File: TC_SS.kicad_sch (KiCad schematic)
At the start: 25 parts, among them J1 Conn_01x08_Pin, J2 Conn_01x08_Pin, Q1 IPW60R099P6XKSA1, Q2 IPW60R099P6XKSA1, Q3 IPW60R099P6XKSA1, Q4 IPW60R099P6XKSA1

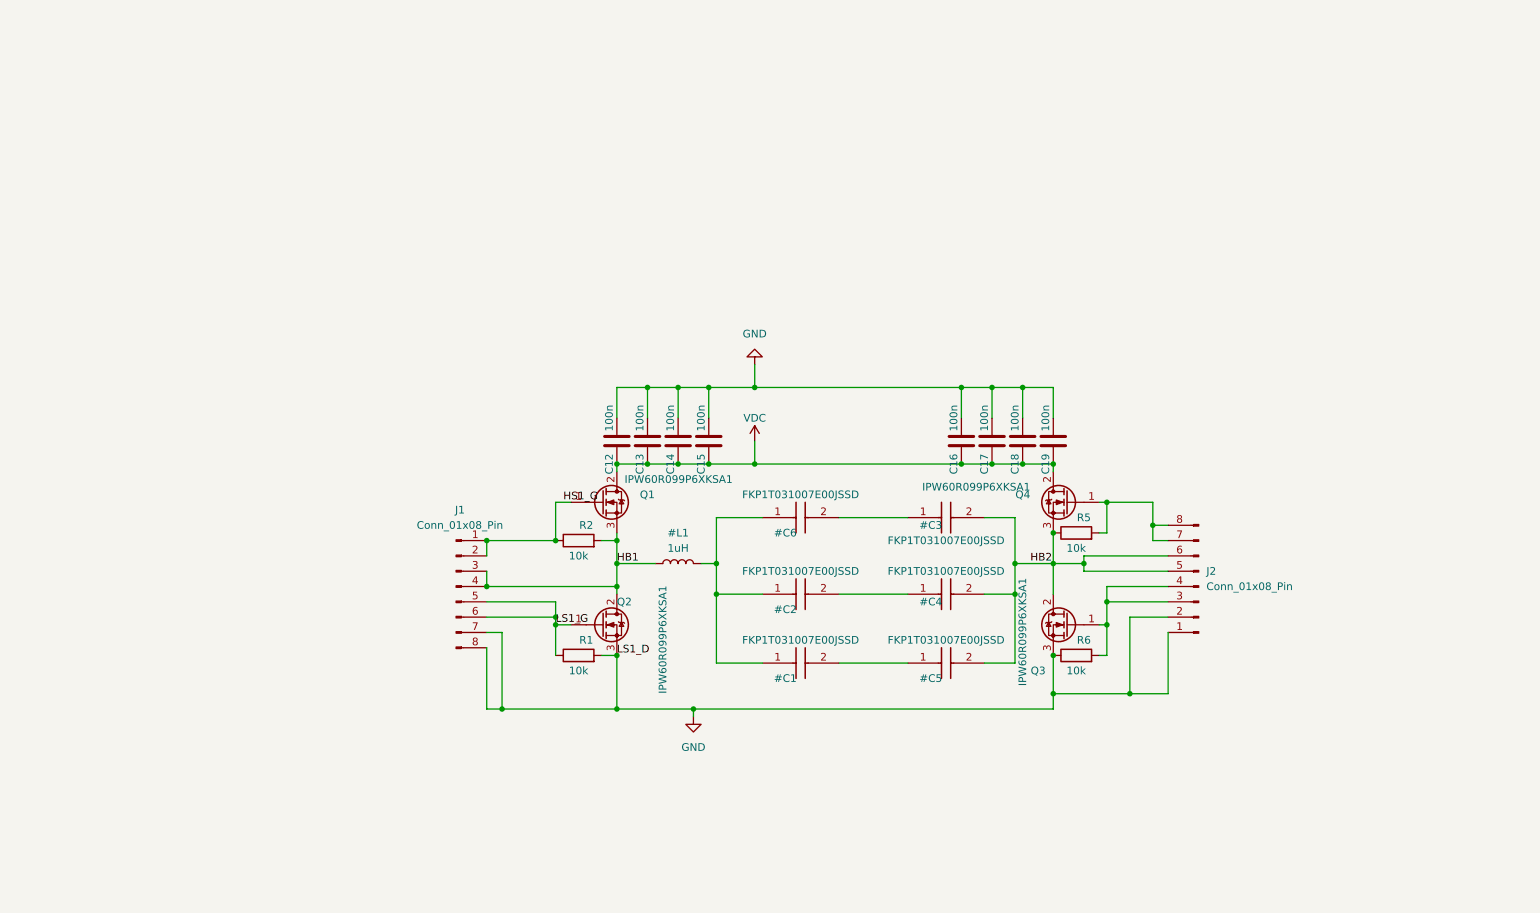
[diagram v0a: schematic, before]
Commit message: Update basically everything
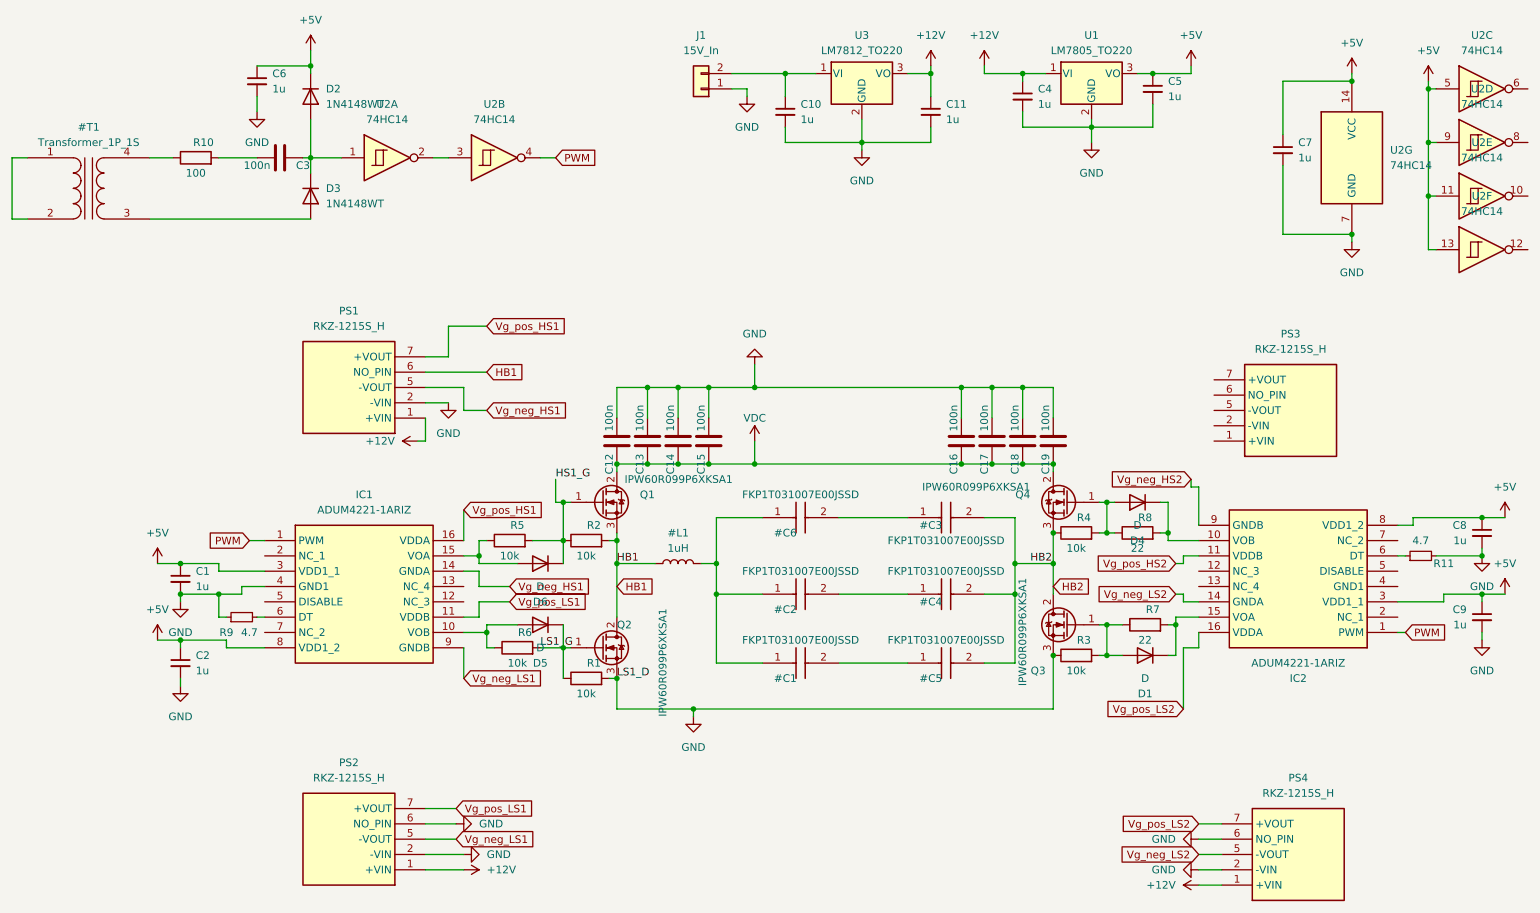
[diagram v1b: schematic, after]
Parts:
- removed J1, J2: Conn_01x08_Pin, Connector_PinHeader_2.54mm:PinHeader_1x08_P2.54mm_Vertical, symbol Connector:Conn_01x08_Pin
- added #T1: Transformer_1P_1S, symbol Device:Transformer_1P_1S
- added C1, C10, C11, C2, C4, C5, C6, C7, C8, C9: 1u, Capacitor_SMD:C_0805_2012Metric, symbol Device:C_Small
- added C3: 100n, Capacitor_SMD:C_2220_5650Metric, symbol Device:C
- added D1, D4, D5, D6: D, PCM_Diode_SMD_AKL:D_PowerDI-123, symbol Device:D
- added D2, D3: 1N4148WT, Diode_SMD:D_SOD-523, symbol Diode:1N4148WT
- added IC1, IC2: ADUM4221-1ARIZ, SamacSys_Parts:SOIC127P1030X264-16N, symbol SamacSys_Parts:ADUM4221-1ARIZ
- added J1: 15V_In, Connector_PinHeader_2.54mm:PinHeader_1x02_P2.54mm_Vertical, symbol Connector_Generic:Conn_01x02
- added PS1, PS2, PS3, PS4: RKZ-1215S_H, symbol:RKZ1215SH, symbol SamacSys_Parts:RKZ-1215S_H
- added R10: 100, Resistor_SMD:R_0805_2012Metric, symbol Device:R
- added R11, R9: 4.7, Resistor_SMD:R_0805_2012Metric, symbol Device:R_Small
- added R3, R4: 10k, Resistor_SMD:R_0805_2012Metric, symbol Device:R
- added R7, R8: 22, Resistor_SMD:R_0805_2012Metric, symbol Device:R
- added U1: LM7805_TO220, Package_TO_SOT_THT:TO-220-3_Vertical, symbol Regulator_Linear:LM7805_TO220
- added U2: 74HC14, symbol 74xx:74HC14
- added U3: LM7812_TO220, Package_TO_SOT_THT:TO-220-3_Vertical, symbol Regulator_Linear:LM7812_TO220
- R1, R2, R5, R6: footprint Resistor_SMD:R_1206_3216Metric_Pad1.30x1.75mm_HandSolder -> Resistor_SMD:R_0805_2012Metric
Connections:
- net GND: now also C1.2, C10.2, C11.2, C2.2, C4.2, C5.2, C6.2, C7.2, C8.2, C9.2, IC1.4 (GND1), J1.1 (Pin_1), PS1.2 (-VIN), PS2.2 (-VIN), PS2.6 (NO_PIN), PS4.2 (-VIN), PS4.6 (NO_PIN), R11.2, R3.1, R9.1, U1.2 (GND), U2.7 (GND), U3.2 (GND); no longer R6.1
- net HB1: now also PS1.6 (NO_PIN)
- net HB2: now also R4.1; no longer R5.1
- net HS1_G: now also R5.2, D6.1 (K)
- net LS1_G: now also R6.2, D5.1 (K)
- net at Q4.1 (G): now also D4.2 (A), R4.2, R8.1; no longer R5.2
- net at Q3.1 (G): now also D1.2 (A), R3.2, R7.1; no longer R6.2
- new net: #T1.4 (SB), R10.1
- new net: C3.2, R10.2
- new net: D4.1 (K), IC2.10 (VOB), R8.2
- new net: D5.2 (A), IC1.10 (VOB), R6.1
- new net: D6.2 (A), IC1.15 (VOA), R5.1
- new net: IC1.6 (DT), R9.2
- new net: C3.1, D2.2 (A), D3.1 (K), U2.1
- new net: D1.1 (K), IC2.15 (VOA), R7.2
- new net: U2.2, U2.3
- new net: IC2.6 (DT), R11.1
- new net: C10.1, J1.2 (Pin_2), U3.1 (VI)
- new net: #T1.3 (SA), D3.2 (A)
- new net: #T1.1 (AA), #T1.2 (AB)
- new net +12V: C11.1, C4.1, PS1.1 (+VIN), PS2.1 (+VIN), PS4.1 (+VIN), U1.1 (VI), U3.3 (VO)
- new net +5V: C1.1, C2.1, C5.1, C6.1, C7.1, C8.1, C9.1, D2.1 (K), IC1.3 (VDD1_1), IC1.8 (VDD1_2), IC2.3 (VDD1_1), IC2.8 (VDD1_2), U1.3 (VO), U2.11, U2.13, U2.14 (VCC), U2.5, U2.9
- new net PWM: IC1.1 (PWM), IC2.1 (PWM), U2.4
- new net Vg_neg_HS1: IC1.14 (GNDA), PS1.5 (-VOUT)
- new net Vg_neg_HS2: IC2.9 (GNDB)
- new net Vg_neg_LS1: IC1.9 (GNDB), PS2.5 (-VOUT)
- new net Vg_neg_LS2: IC2.14 (GNDA), PS4.5 (-VOUT)
- new net Vg_pos_HS1: IC1.16 (VDDA), PS1.7 (+VOUT)
- new net Vg_pos_HS2: IC2.11 (VDDB)
- new net Vg_pos_LS1: IC1.11 (VDDB), PS2.7 (+VOUT)
- new net Vg_pos_LS2: IC2.16 (VDDA), PS4.7 (+VOUT)
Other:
- moved on the sheet: Q2, R2
